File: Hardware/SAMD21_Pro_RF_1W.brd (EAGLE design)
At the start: 53.3 x 40.6 mm, 155 parts, among them J10 AVR_SPI_PROG_3X2TESTPOINTS, J12 JST, J13 U.FL, J14 RFM_DIO, J7 PTH, J9 External On/Off, U1 MCP73831, U2 ADJ3.3, U4 ATSAMD21G, U5 4MB Flash, U6 E19-915MS1W, U7 ADJ5, U8 TXB0108DQSR, U9 TXB0108DQSR, Y1 32.768kHz

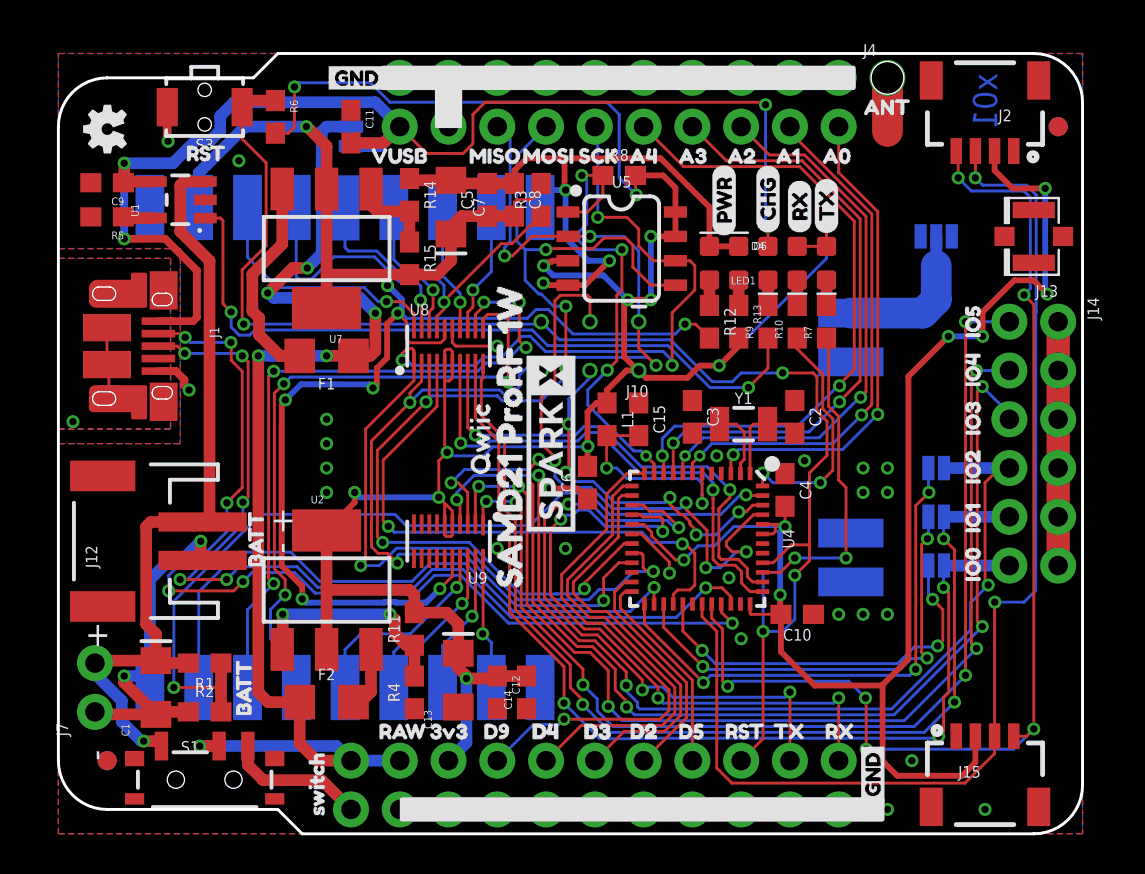
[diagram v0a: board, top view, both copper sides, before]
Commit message: Updates from board review
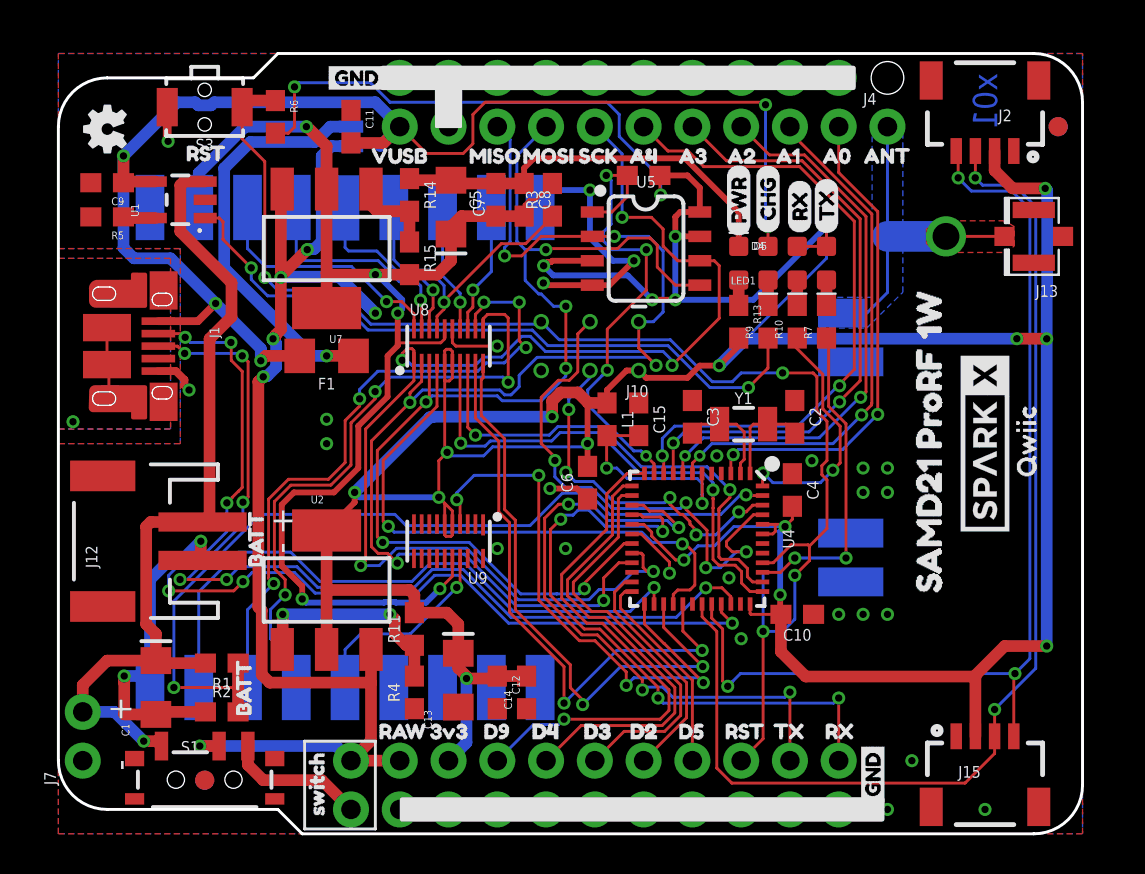
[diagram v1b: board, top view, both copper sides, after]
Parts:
- removed F2: 6V/0.75A, SparkFun-Fuses:1206
- removed J14: RFM_DIO, SparkFun-Connectors:2X6_NOSILK
- removed JP1, JP2: (no value), SparkFun-Jumpers:SMT-JUMPER_2_NO_SILK
- removed JP3: JUMPER-SMT_3_1-NC_PASTE_SILK, SparkFun-Jumpers:SMT-JUMPER_3_1-NC_PASTE_SILK
- removed JP6: JUMPER-SMT_2_NC_PASTE_SILK, SparkFun-Jumpers:SMT-JUMPER_2_NC_PASTE_SILK
- removed LED2: RED, SparkFun-LED:LED-0603
- removed R12: 1k, SparkFun-Resistors:0603
- removed U$54: (no value), ANT:ANT0
- removed U$56: (no value), ufl:U#FL0
- removed U$64, U$75: (no value), buzzard_labels:IO00
- removed U$66, U$76: (no value), buzzard_labels:IO11
- removed U$67, U$77: (no value), buzzard_labels:IO22
- removed U$68, U$78: (no value), buzzard_labels:IO33
- removed U$71, U$79: (no value), buzzard_labels:IO44
- removed U$74, U$80: (no value), buzzard_labels:IO55
- D4: value Yellow -> BLUE
- moved U$60 28.4 mm to (50.4, 17.7)
- moved U$51 22.6 mm to (48.3, 20.3)
- moved U$81 21.8 mm to (45.3, 11.4)
- moved FD1 5.18 mm to (7.62, 2.79)
- moved FD3 5.18 mm to (7.62, 2.79)
- moved J7 2.62 mm to (1.27, 3.81)
- moved J4 2.54 mm to (43.2, 36.8)
- moved U$11 2.54 mm to (41.3, 35.3)
- moved U$50 2.54 mm to (45.1, 35.3)
- moved R8 1.27 mm to (30.5, 34.3)
- moved U5 1.27 mm to (30.6, 30.5)
- moved R1 0.89 mm to (8.51, 8.89)
- moved R2 0.89 mm to (8.51, 6.35)
- moved U$63 0.76 mm to (35.4, 31.1)
- moved R3 0.58 mm to (25.7, 33.0)
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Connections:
- removed net ANT_HEADER: J4.1, JP3.1
- removed net DIO0: J14.11, JP6.1, U8.9
- removed net DIO1: J14.9, JP1.1, U8.10
- removed net DIO2: J14.7, JP2.1, U9.4
- removed net DIO3: J14.5, U9.3
- removed net DIO35V: U6.P$4, U9.18
- removed net DIO4: J14.3, U9.2
- removed net DIO45V: U6.P$3, U9.19
- removed net DIO5: J14.1, U9.1
- removed net DIO55V: U6.P$2, U9.20
- removed net N$10: LED2.A, R12.1
- removed net N$3: J13.FEED, JP3.3
- removed net N$4: F2.2, U2.3
- net 5V: no longer R12.2
- net ANT: now also J13.FEED, J4.1; no longer JP3.2
- net D10: now also U8.10; no longer JP1.2
- net D11: now also U9.4; no longer JP2.2
- net GND: no longer J14.10, J14.12, J14.2, J14.4, J14.6, J14.8, LED2.C
- net N$12: now also F1.1, SJ2.2; no longer F1.2, U7.3
- net RAW: now also U2.3, U7.3; no longer F1.1, F2.1
- net RFM_INT: now also U8.9; no longer JP6.2
- net USB_VCC: now also F1.2; no longer SJ2.2
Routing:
- net DIO3: track 59.1 -> 0.00 mm, vias 5 -> 0
- net DIO5: track 56.8 -> 0.00 mm, vias 5 -> 0
- net DIO4: track 55.4 -> 0.00 mm, vias 5 -> 0
- net DIO1: track 53.9 -> 0.00 mm, vias 3 -> 0
- net DIO2: track 53.2 -> 0.00 mm, vias 4 -> 0
- net DIO0: track 52.6 -> 0.00 mm, vias 3 -> 0
- net 3.3V: track 204.0 -> 240.3 mm, vias 20 -> 21
- net 5V: track 100.3 -> 70.2 mm, vias 8 -> 5
- net GND: track 127.1 -> 114.3 mm, vias 31 -> 28
- net RFM_INT: track 20.4 -> 30.8 mm, vias 3 -> 2
- net N$12: track 11.0 -> 21.3 mm, vias 0 -> 1
- net ANT: track 8.04 -> 17.5 mm, vias 0 -> 1
- net DIO35V: track 8.92 -> 0.00 mm, vias 1 -> 0
- net D10: track 23.7 -> 31.2 mm, vias 3 -> 2
- net DIO45V: track 7.43 -> 0.00 mm, vias 1 -> 0
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- added copper zone on layer 1, net ANT
- added copper zone on layer 16, net ANT
